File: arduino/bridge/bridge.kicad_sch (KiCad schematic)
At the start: 3 parts, among them J1 Conn_01x15_Socket, J2 Conn_01x15_Socket, J3 Conn_01x08_Socket

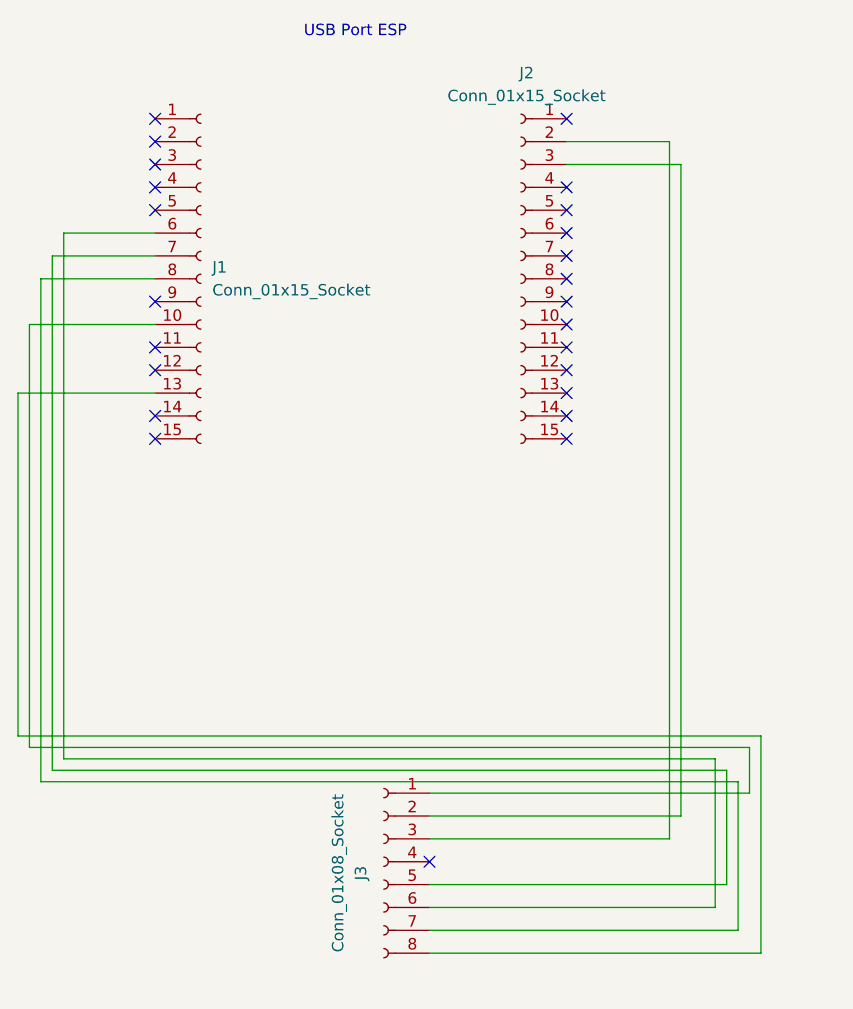
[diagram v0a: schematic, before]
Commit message: bridge edit
pcb and sch edit
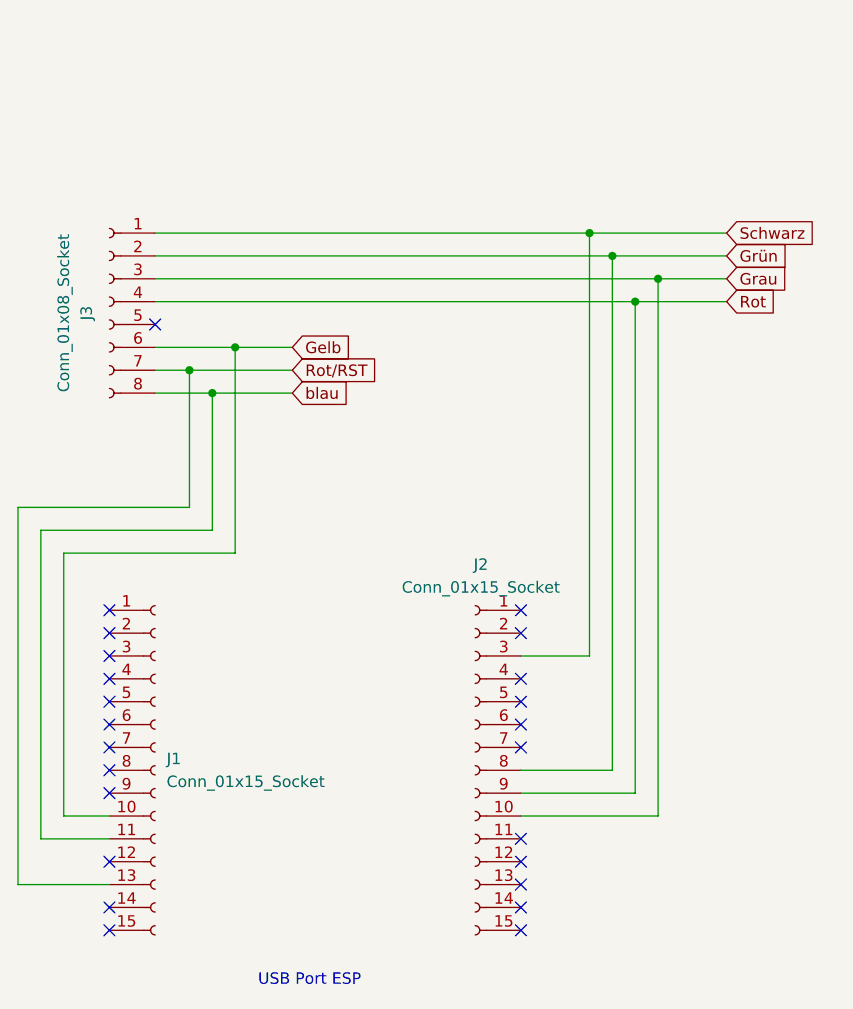
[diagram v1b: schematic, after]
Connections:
- net Gelb: now reaches J1.10 (Pin_10)
- net Gelb: now also J3.6 (Pin_6); no longer J3.1 (Pin_1)
- net Grün: now reaches J3.2 (Pin_2)
- net Grün: now also J2.8 (Pin_8); no longer J2.3 (Pin_3)
- net at J2.2 (Pin_2): no longer J3.3 (Pin_3)
- net Rot: now reaches J3.4 (Pin_4)
- net Rot: now also J2.9 (Pin_9)
- net at J3.5 (Pin_5): no longer J1.7 (Pin_7)
- net at J1.6 (Pin_6): no longer J3.6 (Pin_6)
- net at J1.8 (Pin_8): no longer J3.7 (Pin_7)
- net Rot/RST: now reaches J1.13 (Pin_13)
- net Rot/RST: now also J3.7 (Pin_7); no longer J3.8 (Pin_8)
- net blau: now reaches J1.11 (Pin_11)
- net blau: now also J3.8 (Pin_8)
- net Grau: now reaches J2.10 (Pin_10)
- net Grau: now also J3.3 (Pin_3)
- new net Schwarz: J2.3 (Pin_3), J3.1 (Pin_1)
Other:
- moved on the sheet: J1, J2, J3
